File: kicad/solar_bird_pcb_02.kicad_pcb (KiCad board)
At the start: 2 copper layers, 40 x 24 mm, 8 parts, among them J1 Conn_01x01, J2 Conn_01x01, J3 Conn_01x01, J4 Conn_01x01, J5 Conn_02x03_Odd_Even, U1 ATtiny13V-10PU

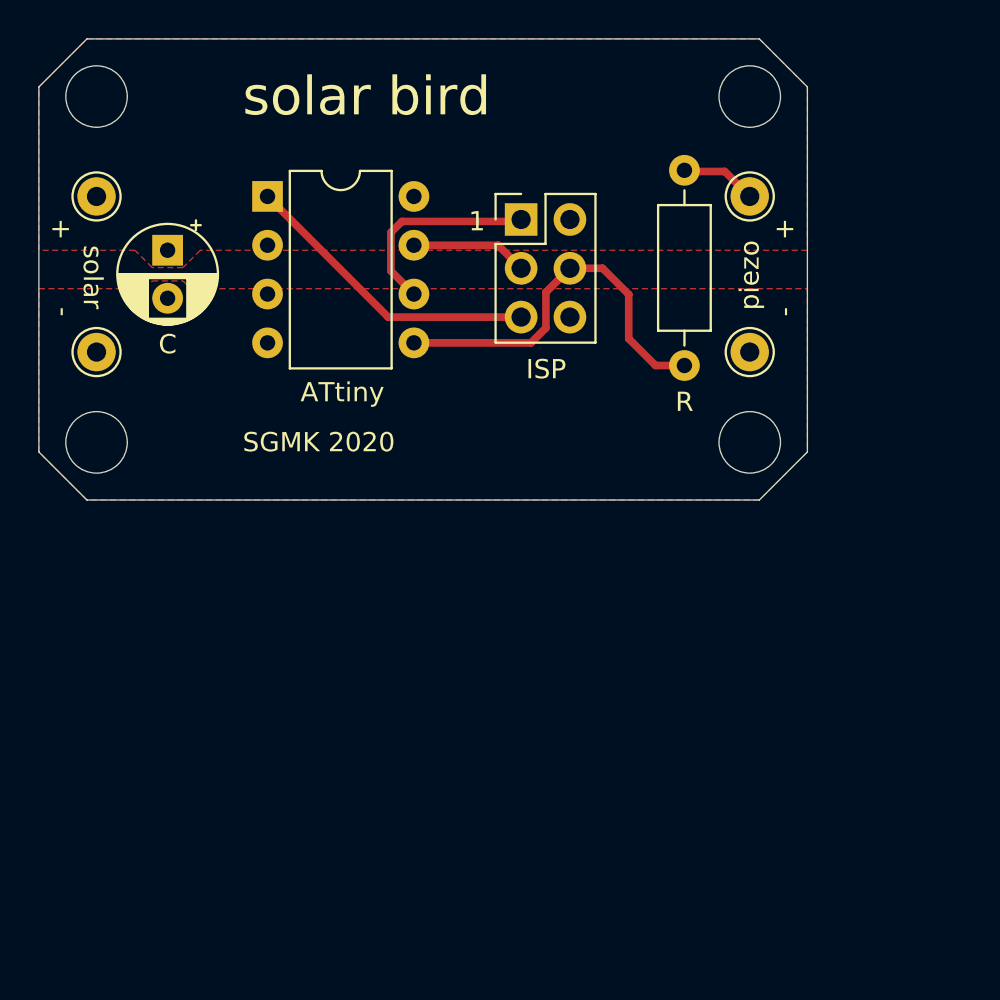
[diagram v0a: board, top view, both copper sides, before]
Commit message: Bird pcb layout
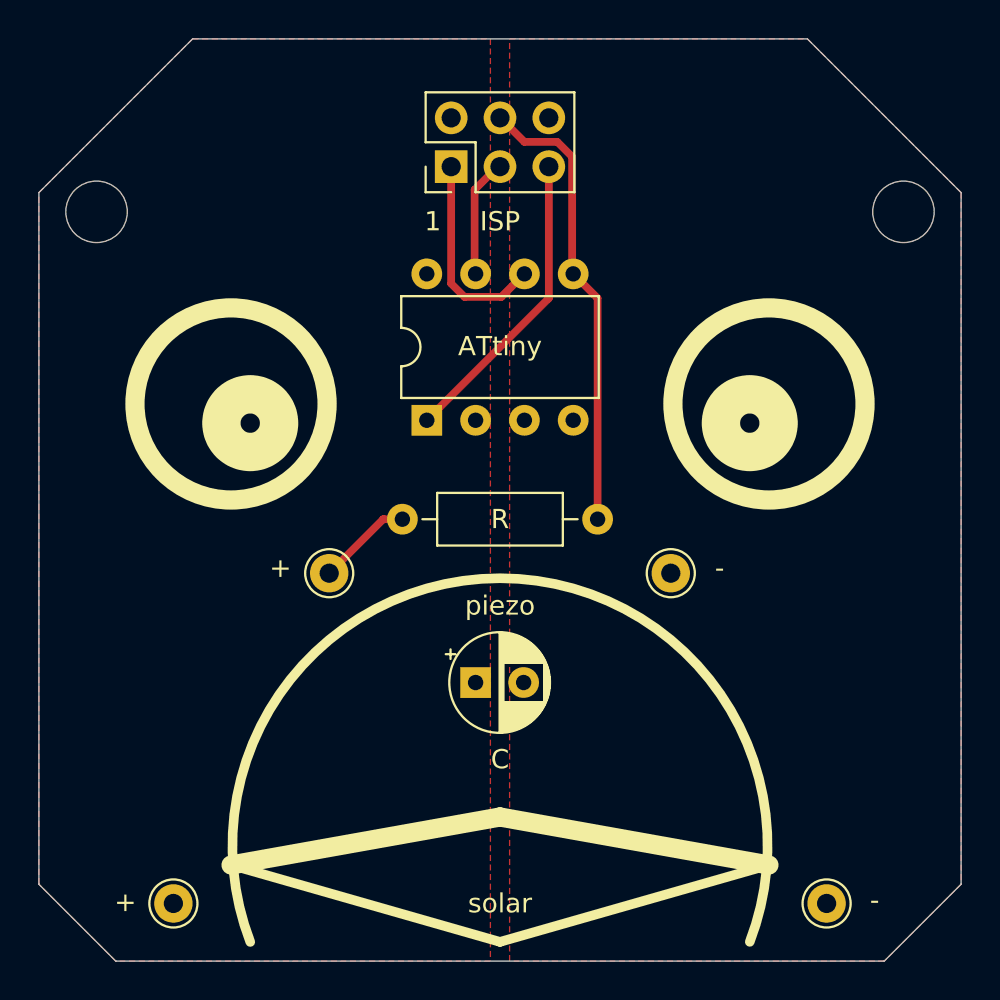
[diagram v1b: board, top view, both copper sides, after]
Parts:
- moved J2 47.6 mm to (141.7, 128.2), turned to 90 degrees
- moved J1 37.0 mm to (107.7, 128.2), turned to 90 degrees
- moved J3 29.4 mm to (115.8, 111.0), turned to 90 degrees
- moved C1 27.6 mm to (123.4, 116.7), turned to 0 degrees
- moved U1 14.3 mm to (120.9, 103.0), turned to 90 degrees
- moved J4 12.2 mm to (133.6, 111.0), turned to 90 degrees
- moved R1 9.19 mm to (129.8, 108.2), turned to 180 degrees
- moved J5 4.56 mm to (122.2, 89.8), turned to 90 degrees
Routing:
- net /MOSI: track 20.2 -> 24.0 mm
- net Net-(J3-Pad1): track 3.96 -> 4.97 mm
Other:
- board size 40 x 24 mm -> 48 x 48 mm
- board text removed: "SGMK 2020"
- board text removed: "solar bird"
